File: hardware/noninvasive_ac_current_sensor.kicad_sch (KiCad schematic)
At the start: 21 parts, among them J6 SJ-3524-SMT, SW1 SW_DIP_x01, U6 MCP4161-xxxx-P, U7 LM358

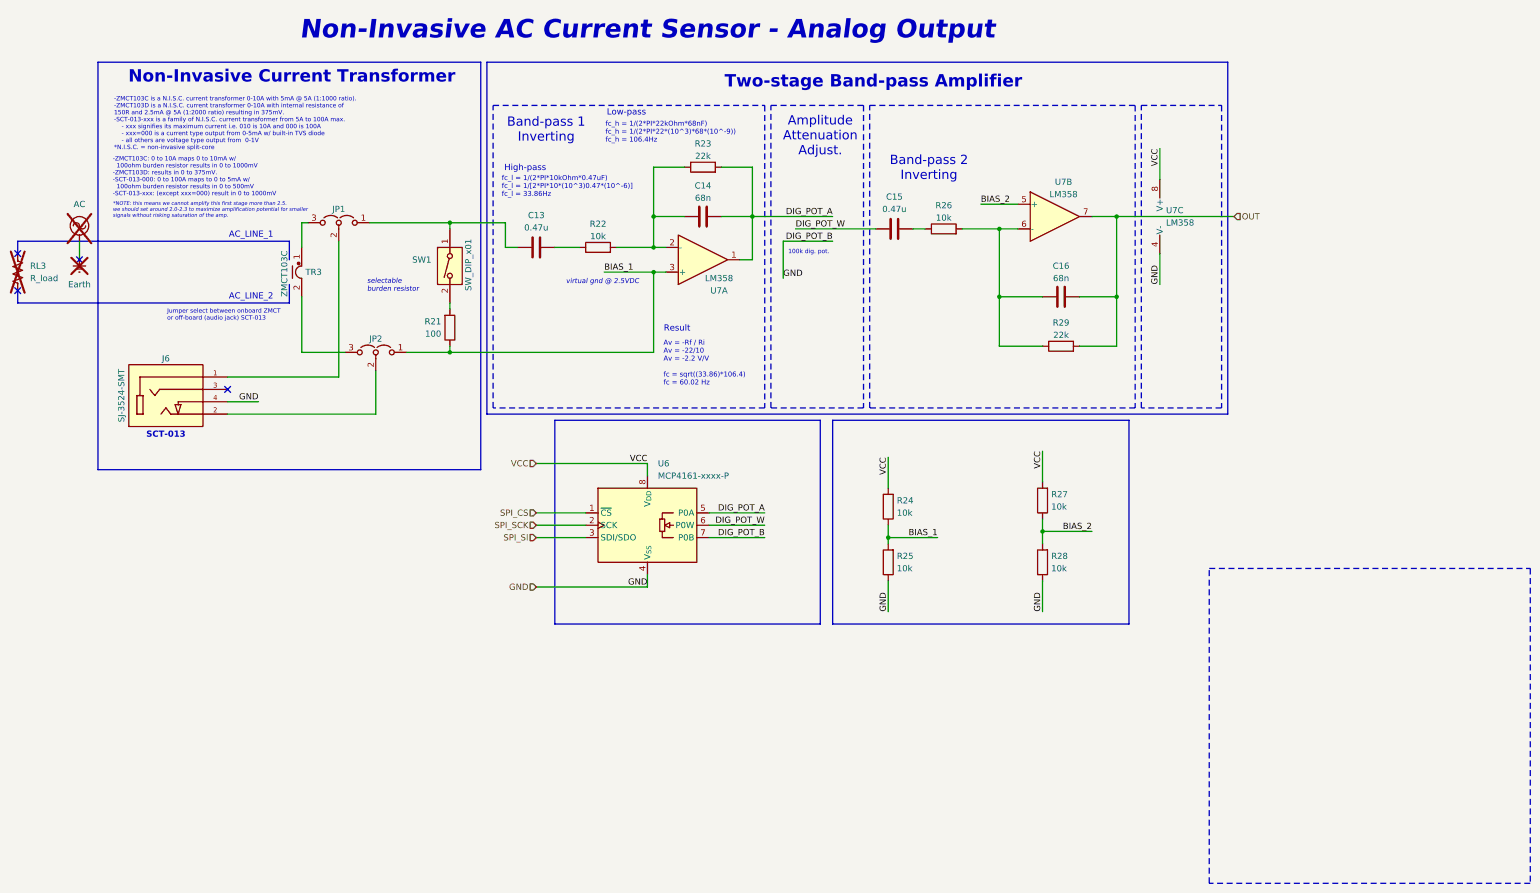
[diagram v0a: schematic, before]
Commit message: finalized pcb
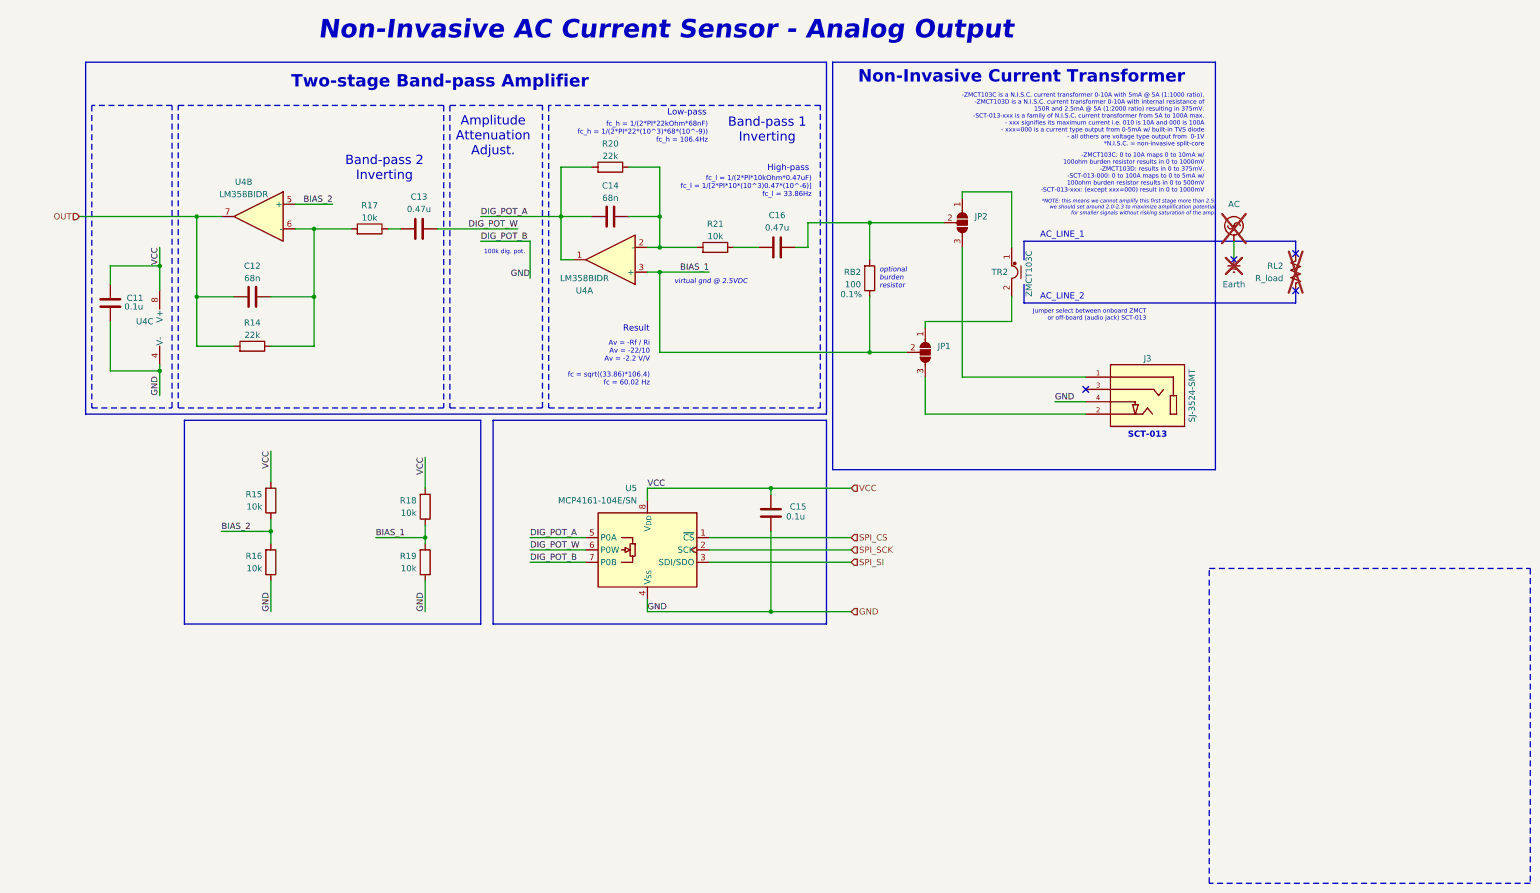
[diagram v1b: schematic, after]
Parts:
- removed JP1, JP2: Jumper_3_Open, symbol Jumper:Jumper_3_Open
- removed R21: 100, symbol Device:R
- removed SW1: SW_DIP_x01, symbol Switch:SW_DIP_x01
- added C11, C15: 0.1u, Capacitor_SMD:C_0805_2012Metric_Pad1.18x1.45mm_HandSolder, symbol Device:C
- added JP1, JP2: SolderJumper_3_Open, Jumper:SolderJumper-3_P2.0mm_Open_TrianglePad1.0x1.5mm, symbol Jumper:SolderJumper_3_Open
- added RB2: 100, Resistor_SMD:R_0805_2012Metric_Pad1.20x1.40mm_HandSolder, symbol Device:R
- C12: renamed from C16; footprint (none) -> Capacitor_SMD:C_0805_2012Metric_Pad1.18x1.45mm_HandSolder
- C13: renamed from C15; footprint (none) -> Capacitor_SMD:C_0805_2012Metric_Pad1.18x1.45mm_HandSolder
- C14: footprint (none) -> Capacitor_SMD:C_0805_2012Metric_Pad1.18x1.45mm_HandSolder
- C16: renamed from C13; footprint (none) -> Capacitor_SMD:C_0805_2012Metric_Pad1.18x1.45mm_HandSolder
- J3: renamed from J6; footprint SJ-3524-SMT:CUI_SJ-3524-SMT -> kml-custom:CUI_SJ-3524-SMT
- R14: renamed from R29; footprint (none) -> Resistor_SMD:R_0805_2012Metric_Pad1.20x1.40mm_HandSolder
- R15: renamed from R27; footprint (none) -> Resistor_SMD:R_0805_2012Metric_Pad1.20x1.40mm_HandSolder
- R16: renamed from R28; footprint (none) -> Resistor_SMD:R_0805_2012Metric_Pad1.20x1.40mm_HandSolder
- R17: renamed from R26; footprint (none) -> Resistor_SMD:R_0805_2012Metric_Pad1.20x1.40mm_HandSolder
- R18: renamed from R24; footprint (none) -> Resistor_SMD:R_0805_2012Metric_Pad1.20x1.40mm_HandSolder
- R19: renamed from R25; footprint (none) -> Resistor_SMD:R_0805_2012Metric_Pad1.20x1.40mm_HandSolder
- R20: renamed from R23; footprint (none) -> Resistor_SMD:R_0805_2012Metric_Pad1.20x1.40mm_HandSolder
- R21: renamed from R22; footprint (none) -> Resistor_SMD:R_0805_2012Metric_Pad1.20x1.40mm_HandSolder
- U4: renamed from U7; value LM358 -> LM358BIDR; footprint (none) -> Package_SO:SOIC-8_3.9x4.9mm_P1.27mm
- U5: renamed from U6; value MCP4161-xxxx-P -> MCP4161-104E/SN; footprint Package_DIP:DIP-8_W7.62mm -> Package_SO:SOIC-8_3.9x4.9mm_P1.27mm
- renumbered RL3 to RL2, TR3 to TR2
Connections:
- net BIAS_1: now also JP1.2 (C), RB2.1
- net GND: now also C11.1, C15.1
- net VCC: now also C11.2, C15.2
- net at C16.1: now also JP2.2 (C), RB2.2
- net at TR2.1: now also JP2.1 (A)
- net at TR2.2: now also JP1.1 (A)
- net at J3.1: now also JP2.3 (B)
- net at J3.2: now also JP1.3 (B)
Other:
- note added: "optional burden resistor"
- note removed: "selectable burden resistor"
- moved on the sheet: C12, C13, C14, C16, J3, R14, R15, R16, R17, R18, R19, R20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
